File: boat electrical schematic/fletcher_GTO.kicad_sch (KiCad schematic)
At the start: 20 parts, among them J1 IGNITION PROBE, K1 FRC2C, K2 FRC2C, K3 DIPxx-1Cxx-51x, K4 DIPxx-1Cxx-51x, M1 PUMP, M2 TRIM, SW1 LIGHT, SW2 HORN, SW3 PUMP, SW5 LIFTING, SW6 LOWERING

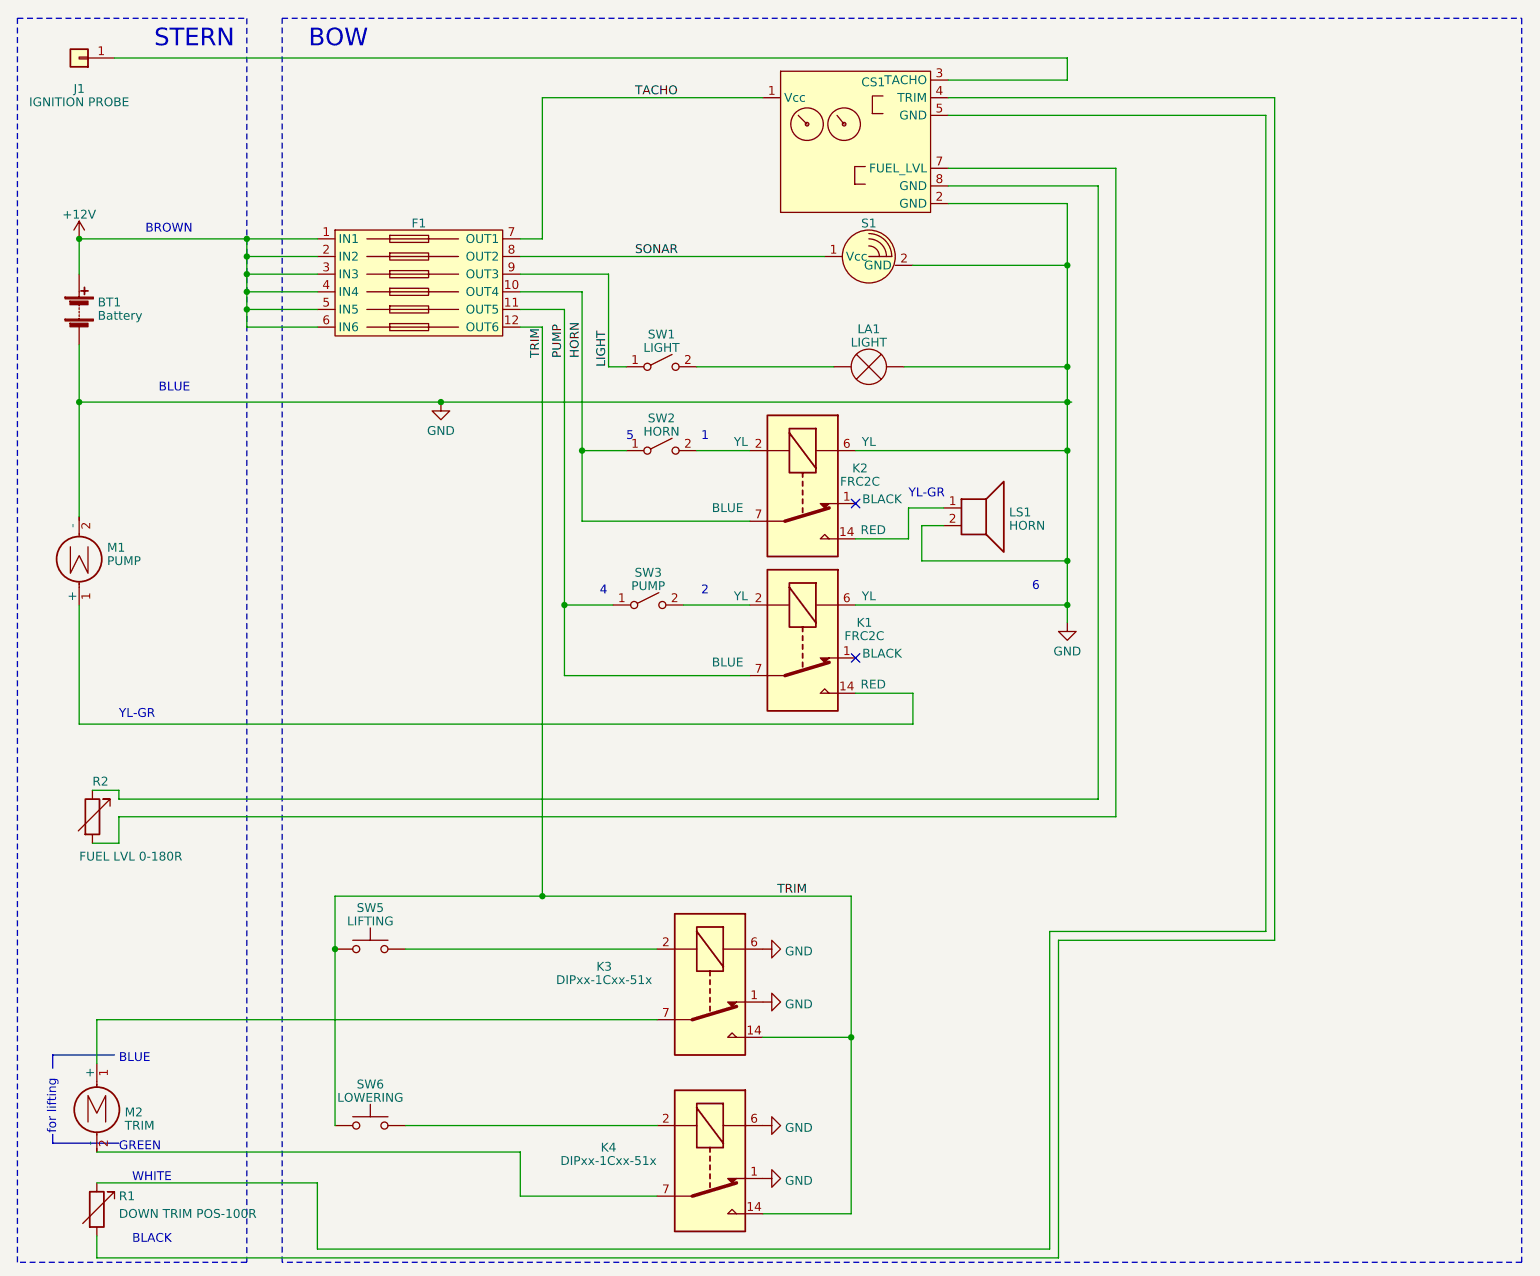
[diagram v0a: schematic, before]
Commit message: add GDT
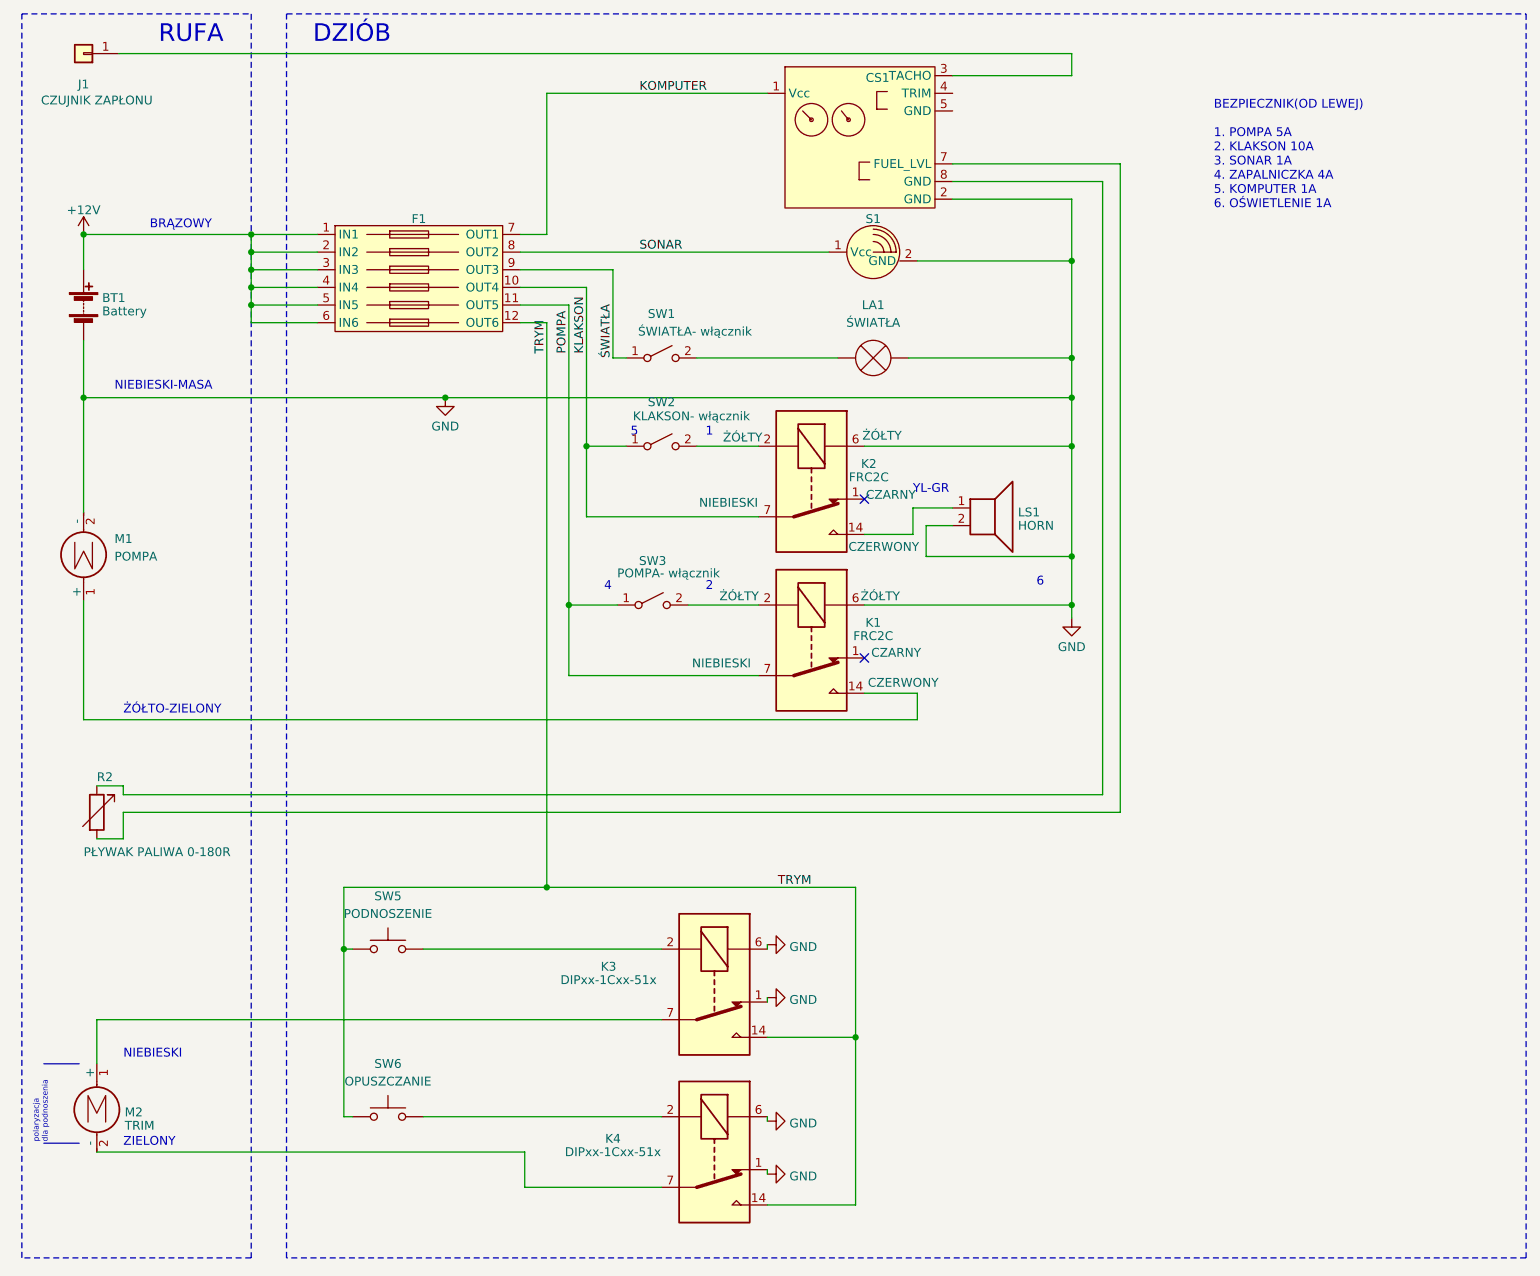
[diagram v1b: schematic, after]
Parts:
- removed R1: DOWN TRIM POS-100R, symbol Device:R_Variable
- J1: value IGNITION PROBE -> CZUJNIK ZAPŁONU
- K1, K2: Field4 YL -> ŻÓŁTY; Field5 YL -> ŻÓŁTY; Field6 BLUE -> NIEBIESKI; Field7 BLACK -> CZARNY; Field8 RED -> CZERWONY
- LA1: value LIGHT -> ŚWIATŁA
- M1: value PUMP -> POMPA
- R2: value FUEL LVL 0-180R -> PŁYWAK PALIWA 0-180R
- SW1: value LIGHT -> ŚWIATŁA- włącznik
- SW2: value HORN -> KLAKSON- włącznik
- SW3: value PUMP -> POMPA- włącznik
- SW5: value LIFTING -> PODNOSZENIE
- SW6: value LOWERING -> OPUSZCZANIE
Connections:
- net HORN renamed KLAKSON
- net LIGHT renamed ŚWIATŁA
- net PUMP renamed POMPA
- net TACHO renamed KOMPUTER
- net TRIM renamed TRYM
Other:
- note added: "BEZPIECZNIK(OD LEWEJ) 1. POMPA 5A 2. KLAKSON 10A 3. SONAR 1A 4. ZAPALNICZKA 4A 5. KOMPUTER 1A 6. OŚWIETLENIE 1A"
- note added: "BRĄZOWY"
- note added: "DZIÓB"
- note added: "NIEBIESKI"
- note added: "NIEBIESKI-MASA"
- note added: "RUFA"
- note added: "ZIELONY"
- note added: "polaryzacja dla podnoszenia"
- note added: "ŻÓŁTO-ZIELONY"
- note removed: "BLACK"
- note removed: "BLUE"
- note removed: "BOW"
- note removed: "BROWN"
- note removed: "GREEN"
- note removed: "STERN"
- note removed: "WHITE"
- note removed: "for lifting"
- moved on the sheet: BT1, CS1, F1, J1, K1, K2, K3, K4, LA1, LS1, M1, R2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
